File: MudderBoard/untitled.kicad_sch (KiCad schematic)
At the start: 9 parts, among them U1 LM51231QRGRRQ1

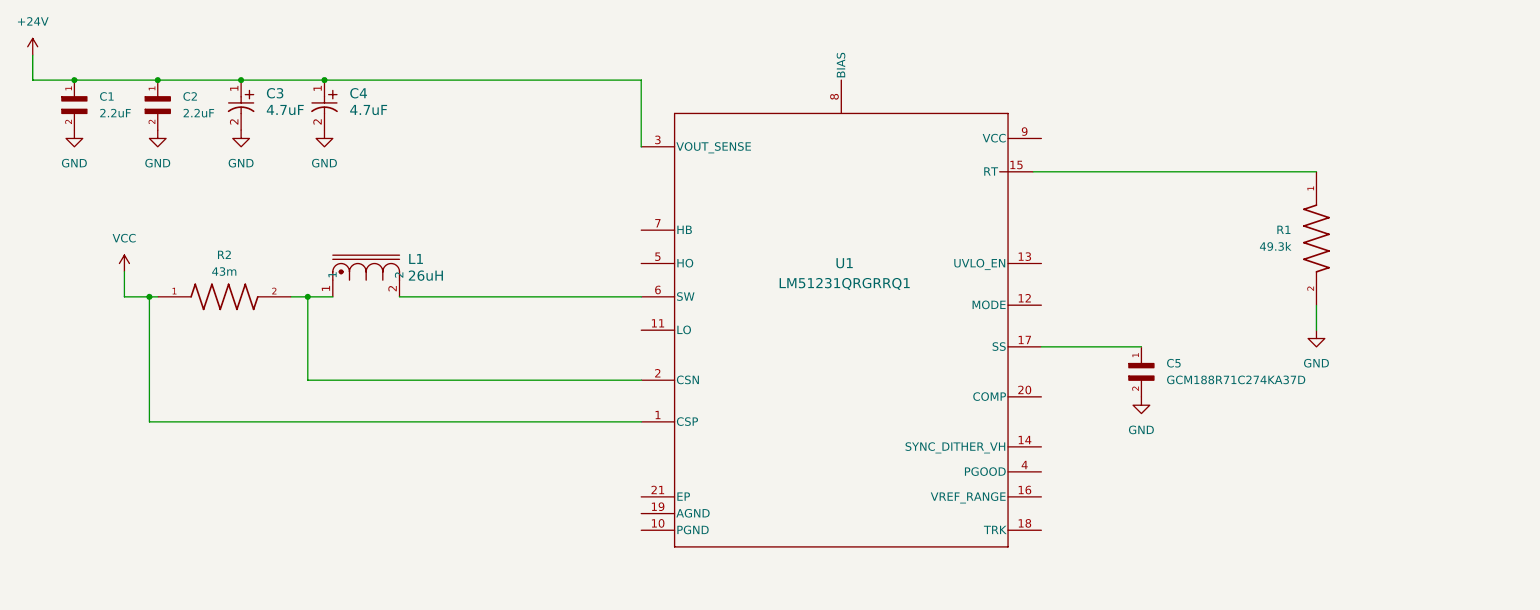
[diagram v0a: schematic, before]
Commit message: schematic_controller update
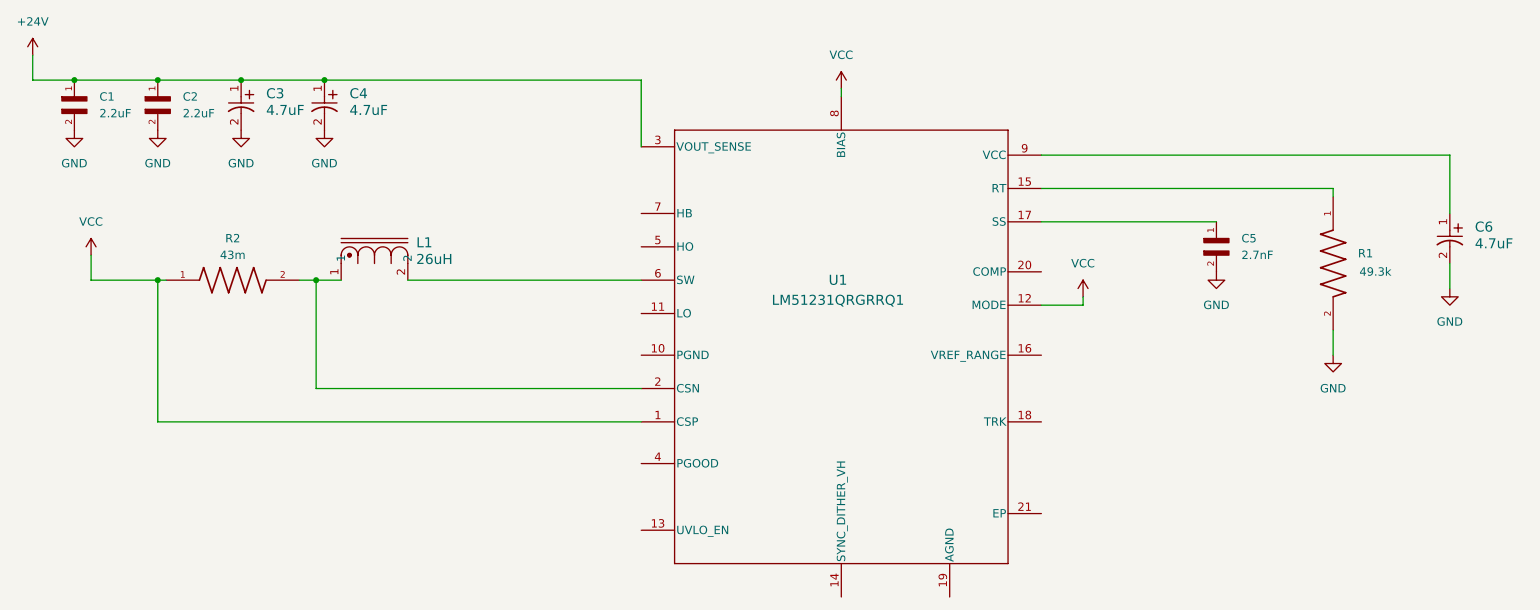
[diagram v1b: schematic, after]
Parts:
- added C6: 4.7uF, TAJB_AVX, symbol TAJB475K035RNJ:TAJB475K035RNJ
- C5: value GCM188R71C274KA37D -> 2.7nF
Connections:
- net GND: now also C6.2
- net VCC: now also U1.12 (MODE), U1.8 (BIAS)
- net at U1.9 (VCC): now also C6.1
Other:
- moved on the sheet: C5, L1, R1, R2, U1
